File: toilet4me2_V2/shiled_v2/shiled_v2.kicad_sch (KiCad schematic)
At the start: 68 parts, among them J1 40HAT, J2 Motor1, J3 Conn_01x01, J4 Conn_01x01, J5 Motor2, J6 Conn_01x01, J7 Conn_01x01, Q1 Q_NMOS_DGS, U1 LM4040DBZ-4.1, U2 MCP3208, U3 AP3012KTR-G1, U4 DHT11, U5 CAT24C32-raspberrypi_hat, U6 MQ-135, U7 MCP47DA1, U8 MQ-136, U9 MQ-137

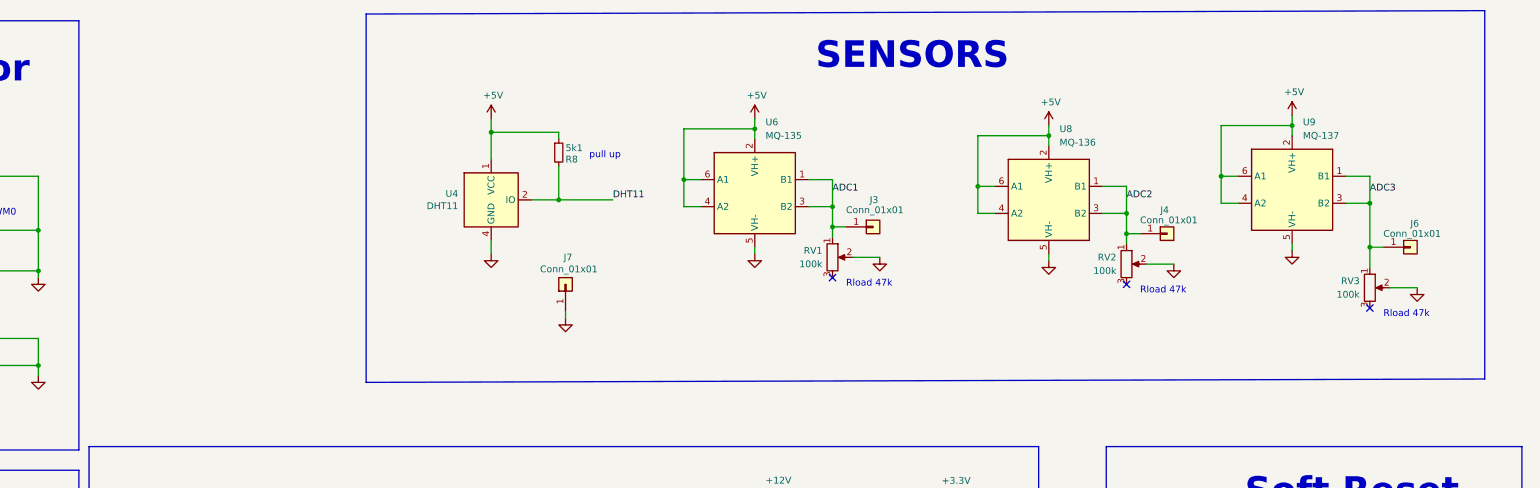
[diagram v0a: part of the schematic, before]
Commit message: t
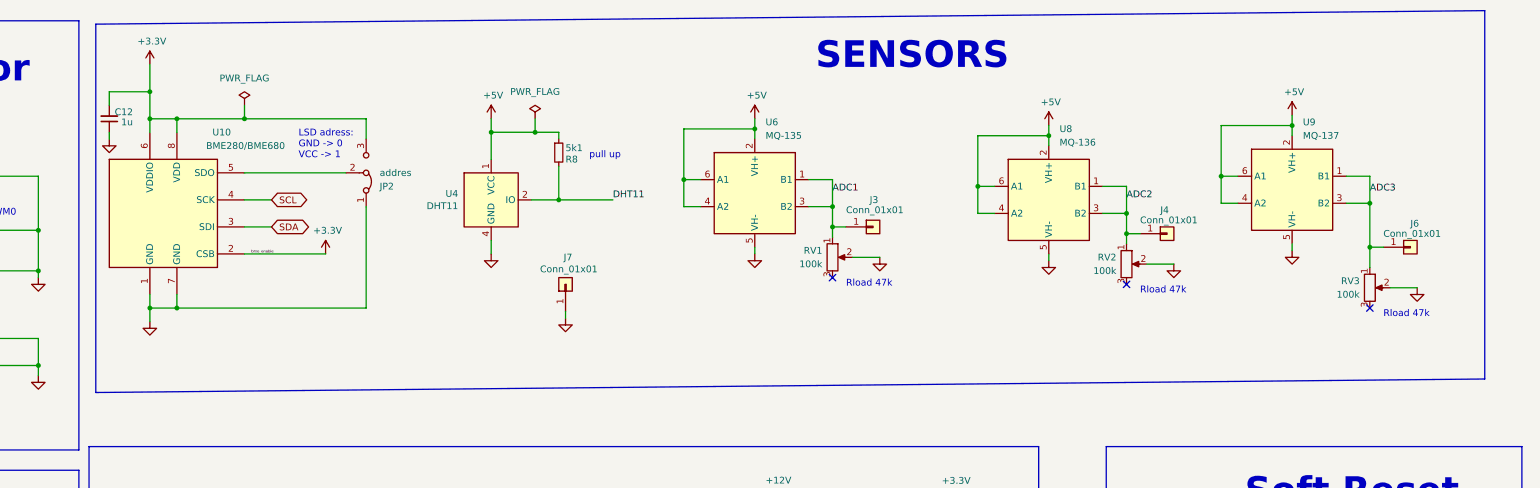
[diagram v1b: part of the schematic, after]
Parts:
- added C12: 1u, Capacitor_SMD:C_0805_2012Metric_Pad1.18x1.45mm_HandSolder, symbol Device:C_Small
- added JP2: addres, Jumper:SolderJumper-3_P1.3mm_Bridged12_Pad1.0x1.5mm, symbol Jumper:Jumper_3_Bridged12
- added U10: BME280/BME680, Package_LGA:Bosch_LGA-8_2.5x2.5mm_P0.65mm_ClockwisePinNumbering, symbol Sensor:BME280
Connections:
- net +3V3: now also C12.2, JP2.3 (B), U10.2 (CSB), U10.6 (VDDIO), U10.8 (VDD)
- net GND: now also C12.1, JP2.1 (A), U10.1 (GND), U10.7 (GND)
- net SCL: now also U10.4 (SCK)
- net SDA: now also U10.3 (SDI)
- new net: JP2.2 (C), U10.5 (SDO)
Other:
- note added: "LSD adress: GND -> 0 VCC -> 1"
